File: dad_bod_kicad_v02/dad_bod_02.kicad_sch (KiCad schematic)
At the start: 65 parts, among them J1 Conn_01x01, J10 Conn_01x03_Male, J12 USB4085-GF-A_REVA4, J13 Conn_01x03_Male, J2 Conn_01x01, J3 Conn_01x01, J4 Conn_01x01, J5 Conn_01x03_Male, J6 Conn_02x15_Odd_Even, J7 BNC5-J-P-GN-RA-BH2D, J8 Conn_01x03_Male, J9 Conn_02x15_Odd_Even, K1 EC2-5NU, K2 EC2-5NU, Q1 2N3904, Q2 2N3904, T1 GT07-110-013, U1 SL1002A600SP

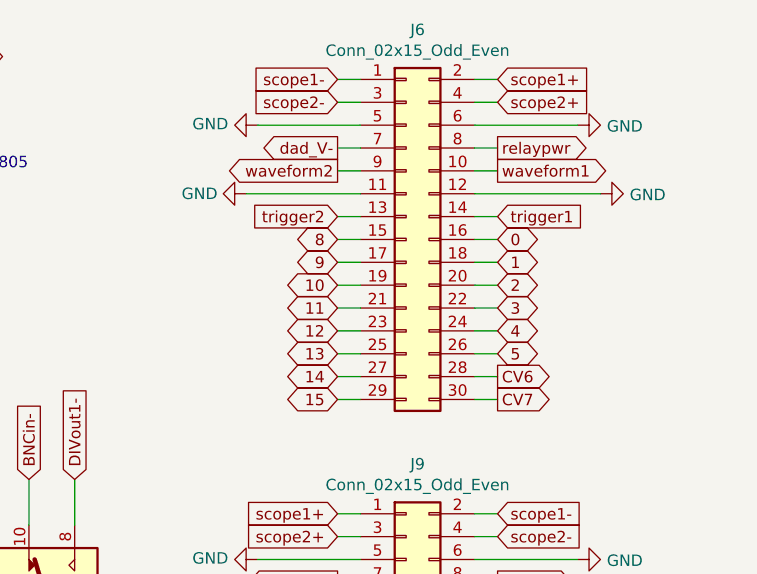
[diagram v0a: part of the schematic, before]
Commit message: Added sketches & iterations
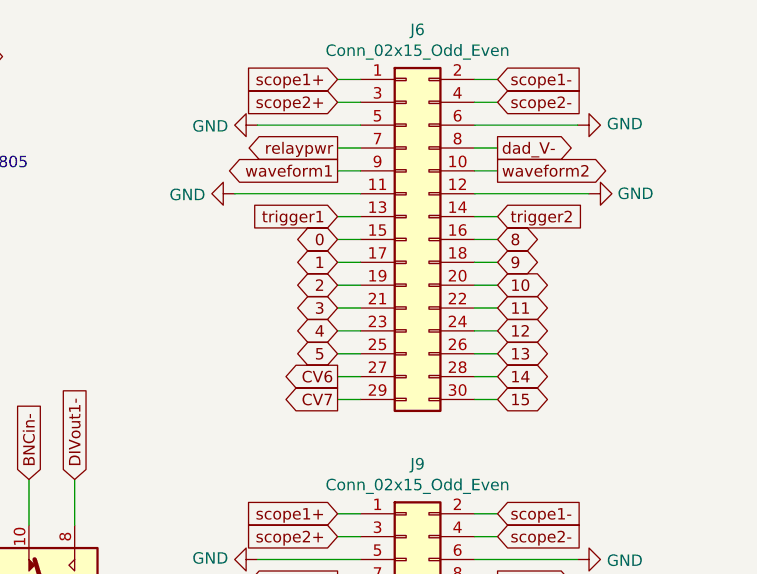
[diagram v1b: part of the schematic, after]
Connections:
- net 0: now also J6.15 (Pin_15); no longer J6.16 (Pin_16)
- net 1: now also J6.17 (Pin_17); no longer J6.18 (Pin_18)
- net 10: now also J6.20 (Pin_20); no longer J6.19 (Pin_19)
- net 11: now also J6.22 (Pin_22); no longer J6.21 (Pin_21)
- net 12: now also J6.24 (Pin_24); no longer J6.23 (Pin_23)
- net 13: now also J6.26 (Pin_26); no longer J6.25 (Pin_25)
- net 14: now also J6.28 (Pin_28); no longer J6.27 (Pin_27)
- net 15: now also J6.30 (Pin_30); no longer J6.29 (Pin_29)
- net 2: now also J6.19 (Pin_19); no longer J6.20 (Pin_20)
- net 3: now also J6.21 (Pin_21); no longer J6.22 (Pin_22)
- net 4: now also J6.23 (Pin_23); no longer J6.24 (Pin_24)
- net 5: now also J6.25 (Pin_25); no longer J6.26 (Pin_26)
- net 8: now also J6.16 (Pin_16); no longer J6.15 (Pin_15)
- net 9: now also J6.18 (Pin_18); no longer J6.17 (Pin_17)
- net CV6: now also J6.27 (Pin_27); no longer J6.28 (Pin_28)
- net CV7: now also J6.29 (Pin_29); no longer J6.30 (Pin_30)
- net dad_V-: now also J6.8 (Pin_8); no longer J6.7 (Pin_7)
- net relaypwr: now also J6.7 (Pin_7); no longer J6.8 (Pin_8)
- net scope1+: now also J6.1 (Pin_1); no longer J6.2 (Pin_2)
- net scope1-: now also J6.2 (Pin_2); no longer J6.1 (Pin_1)
- net scope2+: now also J6.3 (Pin_3); no longer J6.4 (Pin_4)
- net scope2-: now also J6.4 (Pin_4); no longer J6.3 (Pin_3)
- net trigger1: now also J6.13 (Pin_13); no longer J6.14 (Pin_14)
- net trigger2: now also J6.14 (Pin_14); no longer J6.13 (Pin_13)
- net waveform1: now also J6.9 (Pin_9); no longer J6.10 (Pin_10)
- net waveform2: now also J6.10 (Pin_10); no longer J6.9 (Pin_9)
